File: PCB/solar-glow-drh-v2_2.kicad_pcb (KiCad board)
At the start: 6 copper layers, 50.8 x 88.9 mm, 53 parts, among them J1 UPDI hdr, Q1 BCP5316MTWG, SW2 LED master, U1 AVR64DD28 (VQFN28), U2 ALD910025SAL, U3 LIS2DH12, U4 TLV431BCDBZR, U5 NT3H2211 NFC

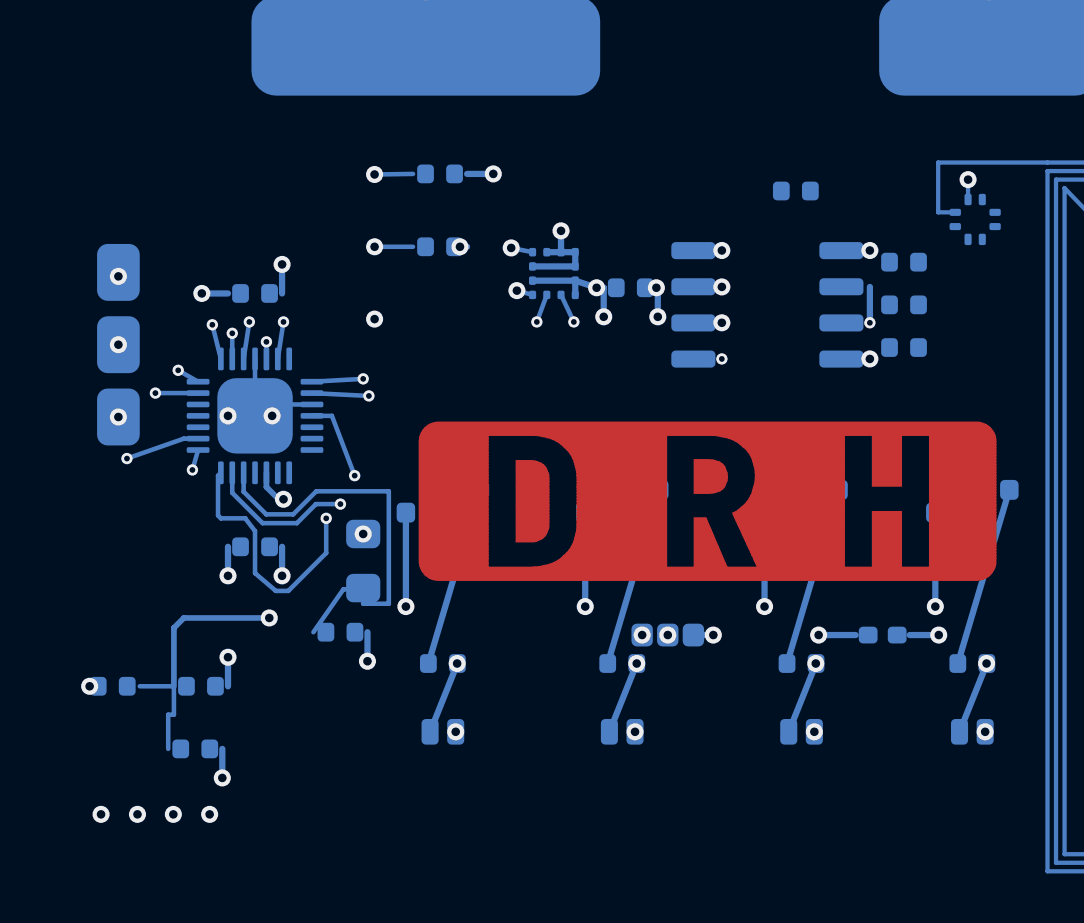
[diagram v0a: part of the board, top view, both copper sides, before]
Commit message: Add files via upload
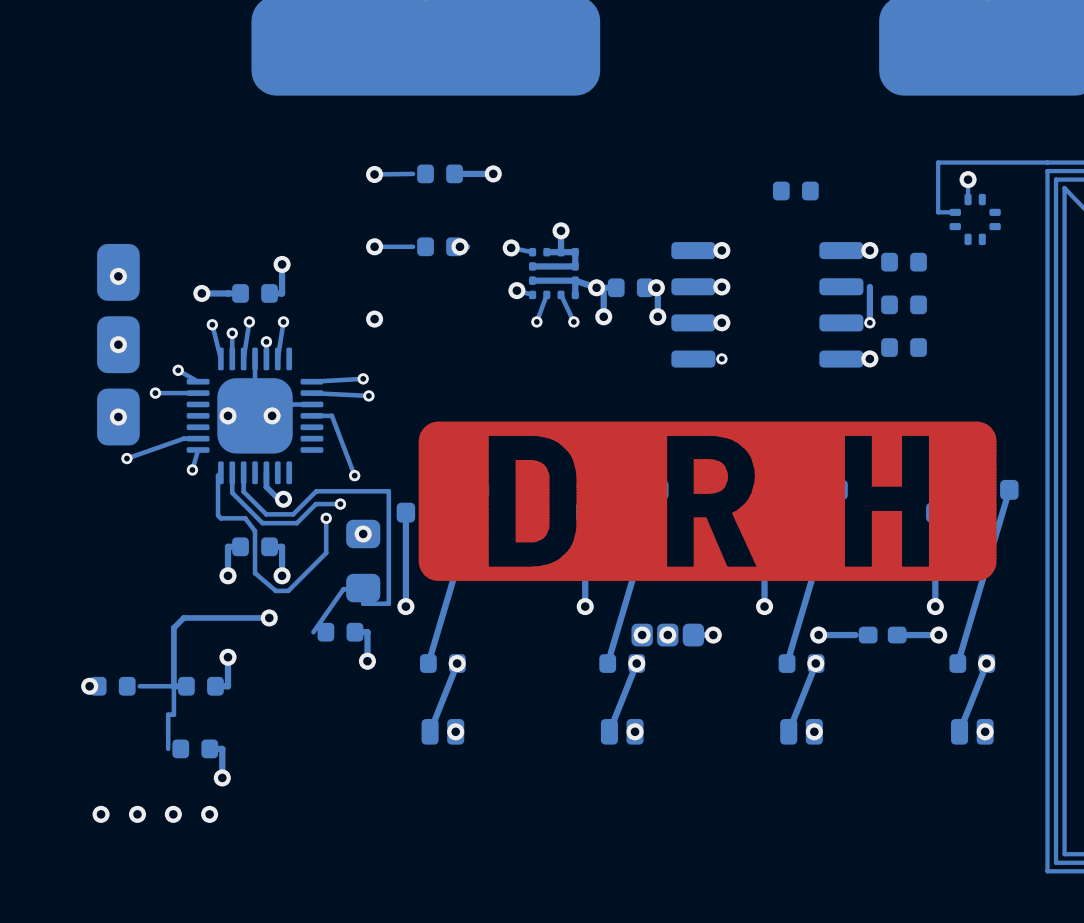
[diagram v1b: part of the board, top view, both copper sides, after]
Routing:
- net VS: track 11.9 -> 14.4 mm
- net GND: track 15.3 -> 17.5 mm
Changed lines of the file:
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@@
+	)
+	(segment
+		(start 13.01 48.5)
+		(end 13.45 48.5)
+		(width 0.22)
+		(layer "B.Cu")
+		(net "GND")
 	)
 	(segment
@@
 	)
 	(segment
+		(start 8.11 50.4)
+		(end 8.55 50.4)
+		(width 0.22)
+		(layer "B.Cu")
+		(net "GND")
+	)
+	(segment
 		(start 20.75 35.65)
 		(end 20.75 35.15)
@@
 	)
 	(segment
+		(start 10.01 45.5)
+		(end 10.45 45.5)
+		(width 0.22)
+		(layer "B.Cu")
+		(net "GND")
+	)
+	(segment
 		(start 10.45 45.5)
 		(end 10.45 46.52)
@@
 	)
 	(segment
+		(start 10.01 36.6)
+		(end 10.45 36.6)
+		(width 0.22)
+		(layer "B.Cu")
+		(net "GND")
+	)
+	(segment
 		(start 8.35 52.6)
 		(end 8.35 53.62)
+		(width 0.22)
+		(layer "B.Cu")
+		(net "GND")
+	)
+	(segment
+		(start 7.91 52.6)
+		(end 8.35 52.6)
 		(width 0.22)
 		(layer "B.Cu")
@@
 	)
 	(segment
+		(start 22.19 36.4)
+		(end 21.5 36.4)
+		(width 0.22)
+		(layer "B.Cu")
+		(net "VS")
+	)
+	(segment
 		(start 20.75 36.15)
 		(end 21.5 36.4)
@@
 	)
 	(segment
+		(start 16.51 32.4)
+		(end 16.95 32.4)
+		(width 0.22)
+		(layer "B.Cu")
+		(net "VS")
+	)
+	(segment
 		(start 9.9 38.9)
 		(end 9.9 38.3)
@@
 		(start 16.95 34.96)
 		(end 16.51 34.96)
+		(width 0.22)
+		(layer "B.Cu")
+		(net "VS")
+	)
+	(segment
+		(start 32.06 48.6)
+		(end 32.5 48.6)
+		(width 0.22)
+		(layer "B.Cu")
+		(net "VS")
+	)
+	(segment
+		(start 8.99 36.6)
+		(end 8.55 36.6)
+		(width 0.22)
+		(layer "B.Cu")
+		(net "VS")
+	)
+	(segment
+		(start 8.99 45.5)
+		(end 8.55 45.5)
 		(width 0.22)
 		(layer "B.Cu")
@@
 		(net "VSENSE")
 	)
+	(segment
+		(start 7.09 50.4)
+		(end 6.65 50.4)
+		(width 0.22)
+		(layer "B.Cu")
+		(net "VSENSE")
+	)
